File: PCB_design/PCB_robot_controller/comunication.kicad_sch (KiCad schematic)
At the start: 3 parts, among them U2 MAX485E

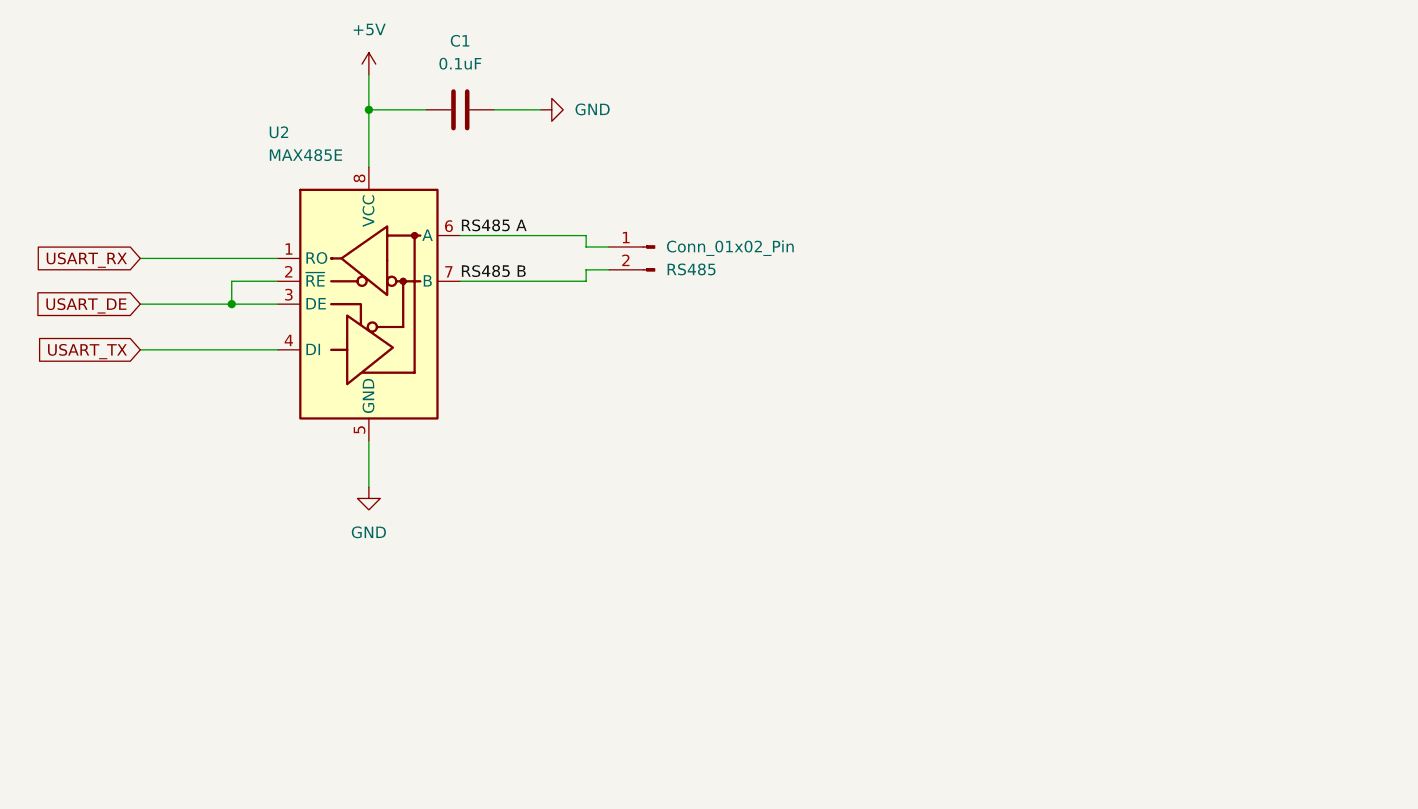
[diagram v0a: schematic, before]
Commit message: pcb to production
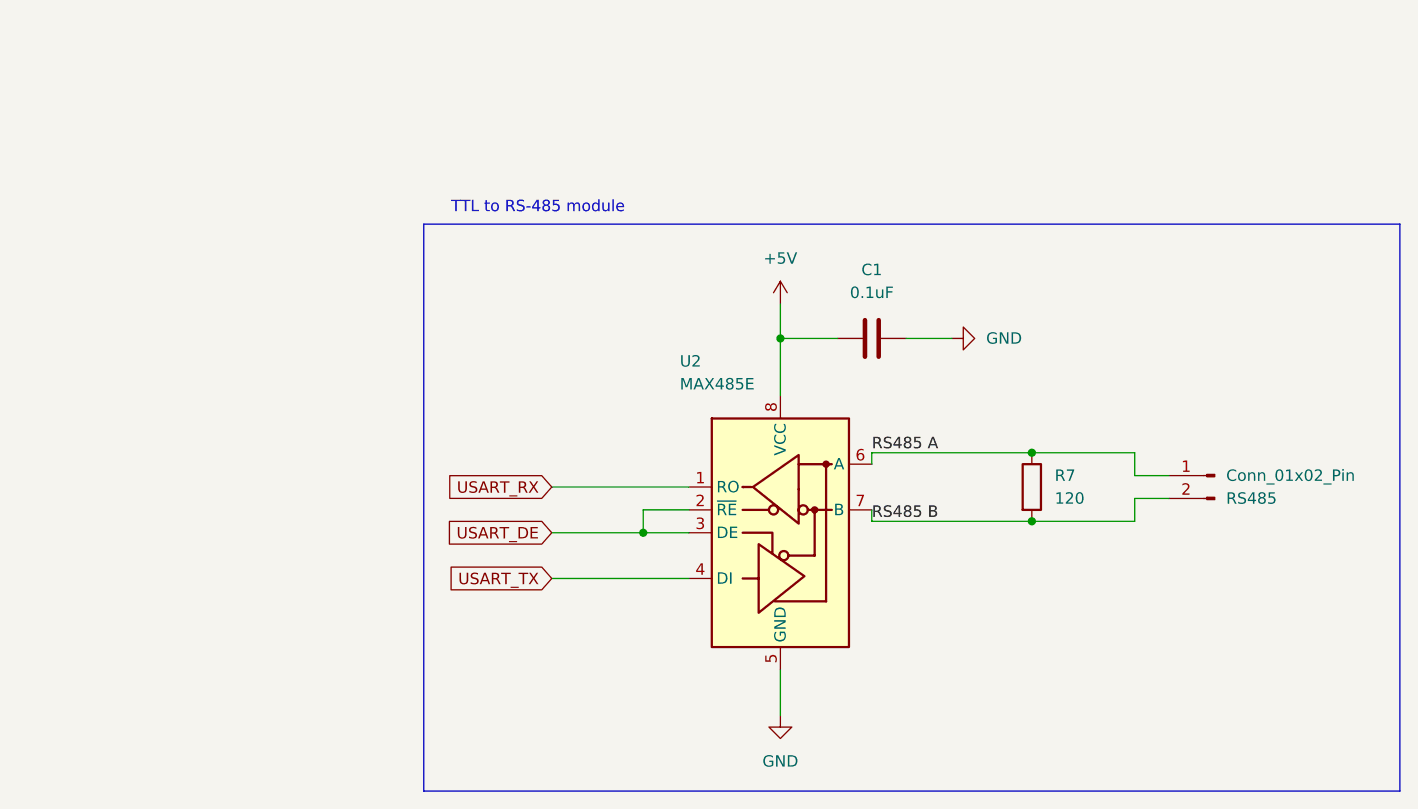
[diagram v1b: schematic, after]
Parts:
- added R7: 120, Resistor_SMD:R_0805_2012Metric, symbol Device:R
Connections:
- net RS485 A: now also R7.1
- net RS485 B: now also R7.2
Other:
- note added: "TTL to RS-485 module"
- moved on the sheet: C1, RS485, U2
